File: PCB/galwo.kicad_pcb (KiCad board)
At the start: 2 copper layers, 20 parts, among them J1 Conn_02x20_Odd_Even, J2 Screw_Terminal_01x02, J3 Screw_Terminal_01x02, J4 Screw_Terminal_01x02, J5 Screw_Terminal_01x02, J6 Screw_Terminal_01x02, J7 Screw_Terminal_01x02, P1 Conn_01x03, U1 MCP4922, U2 MCP4922, U3 MCP4922, U4 TL074, U5 TL074, U6 TL074, U7 TL074

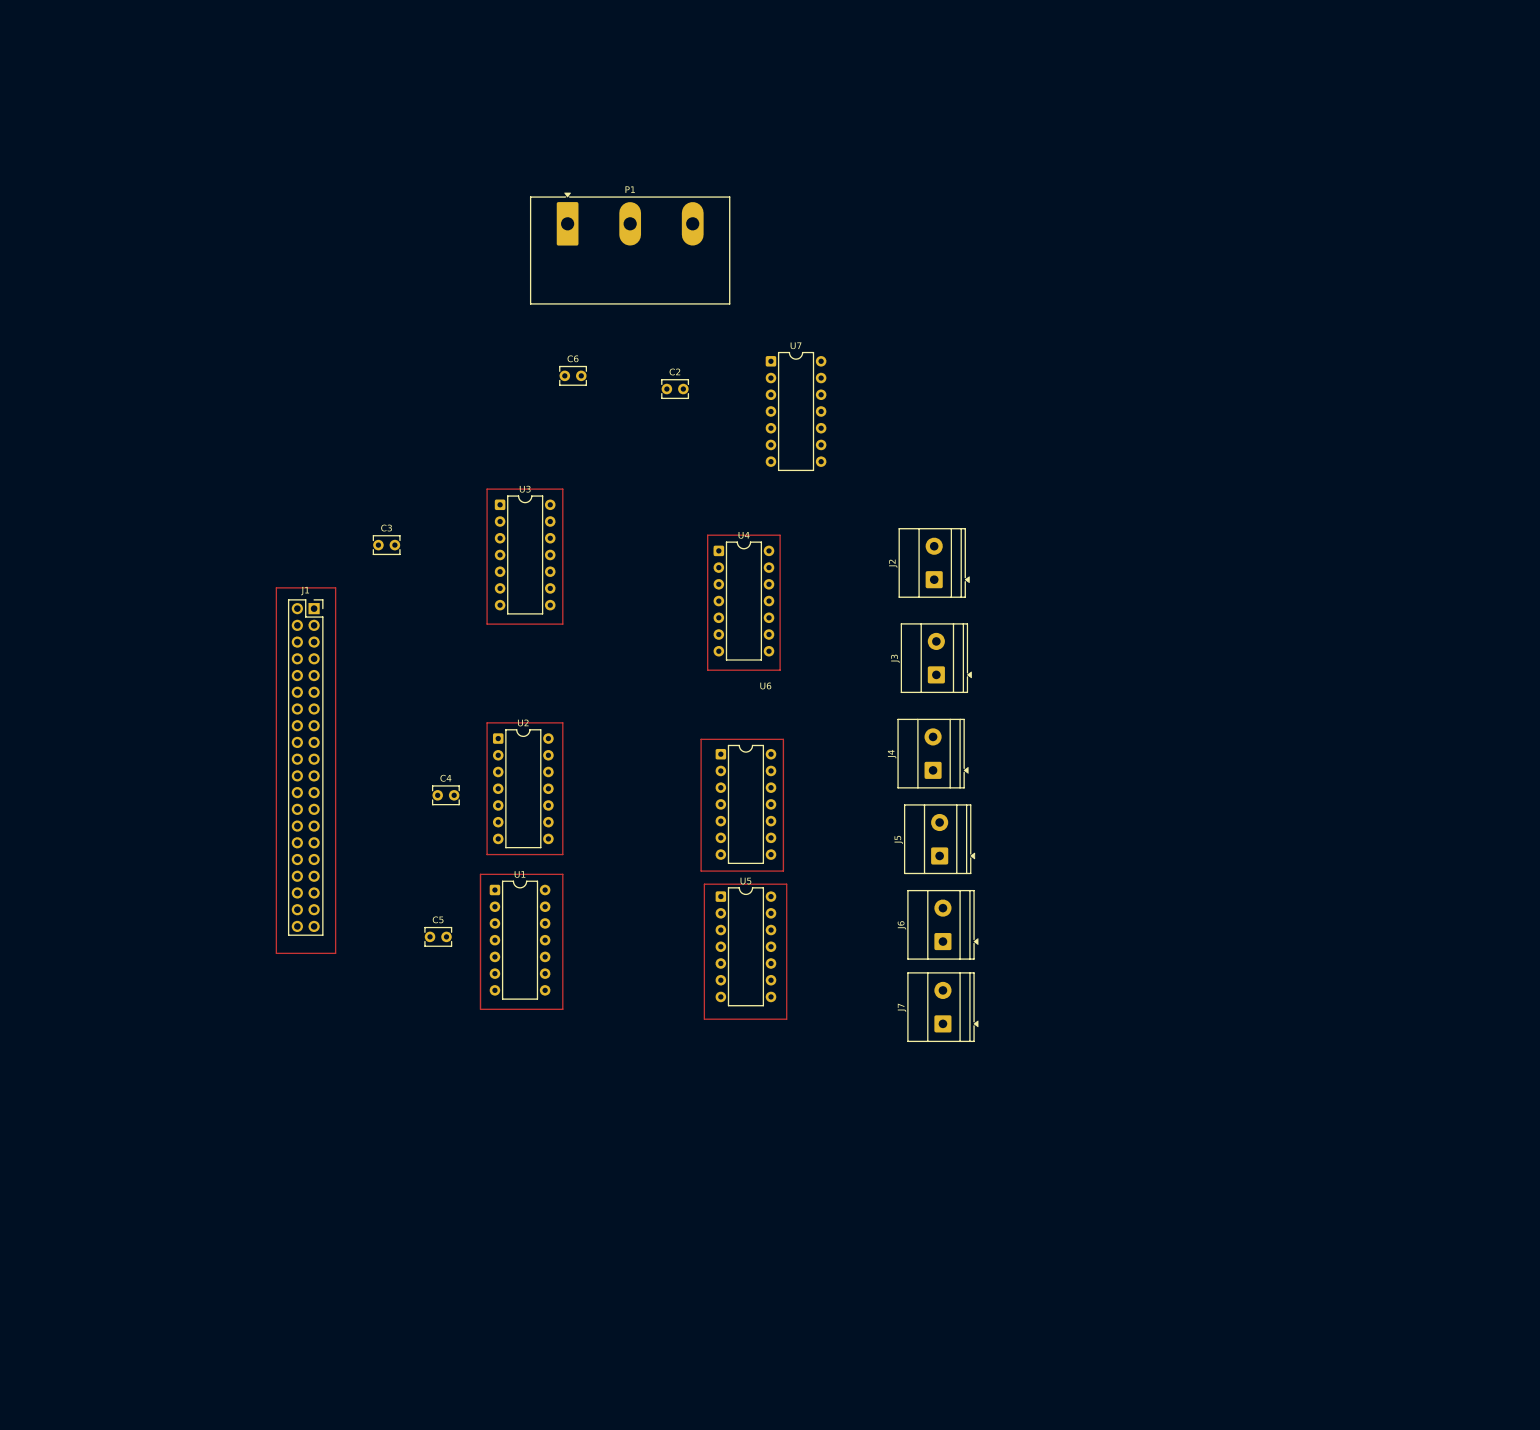
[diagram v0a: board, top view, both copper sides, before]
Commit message: Add files via upload
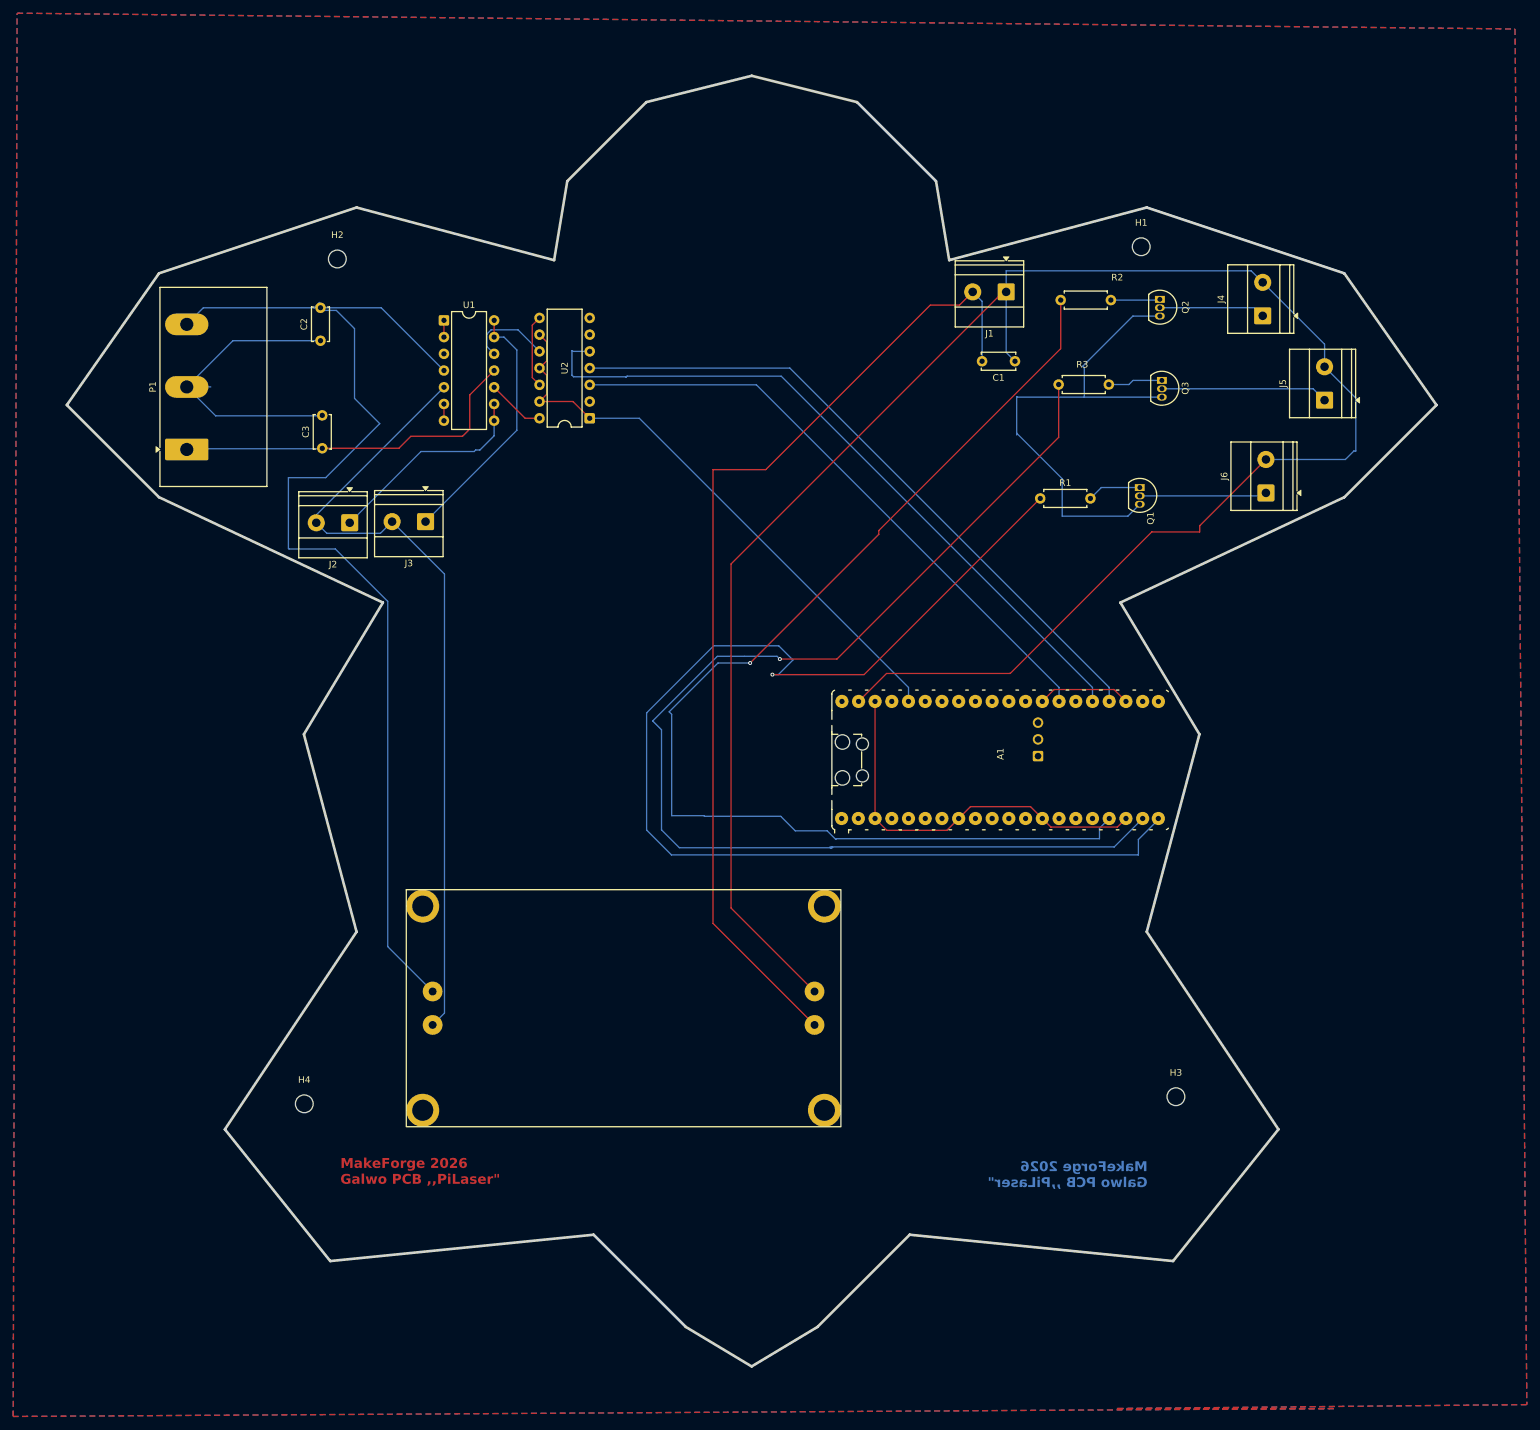
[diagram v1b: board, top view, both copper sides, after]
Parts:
- removed C4, C5, C6: 100nF, Capacitor_THT:C_Disc_D3.8mm_W2.6mm_P2.50mm
- removed U3: MCP4922, Package_DIP:DIP-14_W7.62mm
- removed U4, U5, U6, U7: TL074, Package_DIP:DIP-14_W7.62mm
- added A1: RaspberryPi_Pico_W, proba:RaspberryPi_Pico_W_SMD_HandSolder_tht, F.Cu at (149.7, 112.9)
- added C1: 100nF, Capacitor_THT:C_Disc_D5.0mm_W2.5mm_P5.00mm, F.Cu at (151.9, 52.4)
- added H1: MountingHole, MountingHole:MountingHole_2.7mm_M2.5, F.Cu at (171.1, 35.0)
- added H2: MountingHole, MountingHole:MountingHole_2.7mm_M2.5, F.Cu at (49.0, 36.8)
- added H3: MountingHole, MountingHole:MountingHole_2.7mm_M2.5, F.Cu at (176.4, 164.1)
- added H4: MountingHole, MountingHole:MountingHole_2.7mm_M2.5, F.Cu at (44.0, 165.1)
- added Q1: Q_NPN_BCE, Package_TO_SOT_THT:TO-92L_Inline, F.Cu at (170.9, 71.5)
- added Q2: Q_NPN_BCE, Package_TO_SOT_THT:TO-92L_Inline, F.Cu at (173.9, 43.0)
- added Q3: Q_NPN_BCE, Package_TO_SOT_THT:TO-92L_Inline, F.Cu at (174.2, 55.3)
- added R1: 1k, Resistor_THT:R_Axial_DIN0207_L6.3mm_D2.5mm_P7.62mm_Horizontal, F.Cu at (155.8, 73.2)
- added R2: 1k, Resistor_THT:R_Axial_DIN0207_L6.3mm_D2.5mm_P7.62mm_Horizontal, F.Cu at (158.9, 43.1)
- added R3: 1k, Resistor_THT:R_Axial_DIN0207_L6.3mm_D2.5mm_P7.62mm_Horizontal, F.Cu at (158.6, 55.9)
- C2, C3: footprint Capacitor_THT:C_Disc_D3.8mm_W2.6mm_P2.50mm -> Capacitor_THT:C_Disc_D5.0mm_W2.5mm_P5.00mm
- J1: value Conn_02x20_Odd_Even -> Conn_01x02; footprint Connector_PinSocket_2.54mm:PinSocket_2x20_P2.54mm_Vertical -> TerminalBlock_Phoenix:TerminalBlock_Phoenix_MKDS-1,5-2-5.08_1x02_P5.08mm_Horizontal
- J7: value Screw_Terminal_01x02 -> Conn_02x02_Counter_Clockwise; footprint TerminalBlock_Phoenix:TerminalBlock_Phoenix_MKDS-1,5-2-5.08_1x02_P5.08mm_Horizontal -> proba:Bez_nazwy
- U1: value MCP4922 -> TL074
- moved J1 115.6 mm to (150.6, 41.8), turned to 180 degrees
- moved J5 90.6 mm to (199.0, 58.3)
- moved J2 89.2 mm to (50.9, 76.9), turned to 180 degrees
- moved U1 86.9 mm to (65.2, 46.2)
- moved J4 85.3 mm to (189.6, 45.5)
- moved J6 83.9 mm to (190.1, 72.4)
- moved J3 81.0 mm to (62.4, 76.7), turned to 180 degrees
- moved P1 67.2 mm to (26.2, 65.8), turned to 90 degrees
- moved C2 53.1 mm to (46.5, 49.2), turned to 90 degrees
- moved U2 50.6 mm to (87.4, 61.0), turned to 180 degrees
- moved J7 48.6 mm to (92.5, 150.6), turned to 0 degrees
- moved C3 17.0 mm to (46.7, 65.6), turned to 90 degrees
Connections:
- C2 pad 1: Net-(J1-Pin_1) -> GND
- C2 pad 2: Net-(J1-Pin_6) -> /15V
- C3 pad 1: Net-(J1-Pin_1) -> /-15V
- C3 pad 2: Net-(J1-Pin_6) -> GND
- J1 pad 1: Net-(J1-Pin_1) -> Net-(A1-VSYS)
- J1 pad 2: unconnected-(J1-Pin_2-Pad2) -> GND
- J2 pad 2: Net-(J1-Pin_6) -> GND
- J3 pad 2: Net-(J1-Pin_6) -> GND
- J4 pad 2: Net-(J1-Pin_6) -> Net-(A1-VSYS)
- J5 pad 2: Net-(J1-Pin_6) -> Net-(A1-VSYS)
- J6 pad 2: Net-(J1-Pin_6) -> Net-(A1-VSYS)
- J7 pad 1: Net-(J7-Pin_1) -> GND
- J7 pad 2: Net-(J1-Pin_6) -> /15V
- P1 pad 1: Net-(P1-Pin_1) -> /-15V
- P1 pad 2: Net-(J1-Pin_6) -> GND
- P1 pad 3: Net-(P1-Pin_3) -> /15V
- U1 pad 1: Net-(J1-Pin_1) -> Net-(U1A--)
- U1 pad 10: Net-(U1-VB) -> Net-(U1C-+)
- U1 pad 11: Net-(J1-Pin_1) -> /-15V
- U1 pad 12: Net-(J1-Pin_6) -> Net-(U1D-+)
- U1 pad 13: Net-(J1-Pin_1) -> Net-(J3-Pin_1)
- U1 pad 14: Net-(U1-VA) -> Net-(J3-Pin_1)
- U1 pad 2: unconnected-(U1-NC-Pad2) -> Net-(U1A--)
- U1 pad 3: Net-(J1-Pin_26) -> GND
- U1 pad 4: Net-(J1-Pin_23) -> /15V
- U1 pad 5: Net-(J1-Pin_19) -> GND
- U1 pad 6: unconnected-(U1-NC-Pad6) -> Net-(U1B--)
- U1 pad 7: unconnected-(U1-NC-Pad7) -> Net-(U1B--)
- U1 pad 8: Net-(J1-Pin_6) -> Net-(J2-Pin_1)
- U1 pad 9: Net-(J1-Pin_1) -> Net-(J2-Pin_1)
- U2 pad 1: Net-(J1-Pin_1) -> Net-(A1-3V3)
- U2 pad 10: Net-(U2-VB) -> Net-(U1D-+)
- U2 pad 11: Net-(J1-Pin_1) -> Net-(A1-3V3)
- U2 pad 12: Net-(J1-Pin_6) -> GND
- U2 pad 13: Net-(J1-Pin_1) -> Net-(A1-3V3)
- U2 pad 14: Net-(U2-VA) -> Net-(U1C-+)
- U2 pad 3: Net-(J1-Pin_28) -> Net-(A1-GPIO21)
- U2 pad 4: Net-(J1-Pin_23) -> Net-(A1-GPIO18)
- U2 pad 5: Net-(J1-Pin_19) -> Net-(A1-GPIO19)
- U2 pad 8: Net-(J1-Pin_6) -> GND
- U2 pad 9: Net-(J1-Pin_1) -> Net-(A1-3V3)
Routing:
- net GND: track 0.00 -> 484.6 mm
- net Net-(A1-VSYS): track 0.00 -> 306.3 mm
- net Net-(A1-GPIO15): track 0.00 -> 184.0 mm, vias 0 -> 1
- net Net-(A1-GPIO14): track 0.00 -> 181.8 mm, vias 0 -> 1
- net Net-(A1-GPIO13): track 0.00 -> 176.1 mm, vias 0 -> 1
- net /15V: track 0.00 -> 176.0 mm
- net Net-(A1-GPIO19): track 0.00 -> 107.4 mm
- net Net-(A1-GPIO18): track 0.00 -> 101.1 mm
- net Net-(A1-GPIO21): track 0.00 -> 92.4 mm
- net Net-(A1-3V3): track 0.00 -> 88.1 mm
- net /-15V: track 0.00 -> 54.7 mm
- net Net-(J3-Pin_1): track 0.00 -> 38.6 mm
- net Net-(J2-Pin_1): track 0.00 -> 32.2 mm
- net Net-(J5-Pin_1): track 0.00 -> 25.4 mm
- net Net-(J6-Pin_1): track 0.00 -> 19.3 mm
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- added copper zone on B.Cu, net GND
- added copper zone on F.Cu, net GND
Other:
- board outline added: 208 x 196 mm
- board text added: "Blue"
- board text added: "Green"
- board text added: "MakeForge 2026 Galwo PCB ,,PiLaser{dblquote}"
- board text added: "Os X"
- board text added: "Os Y"
- board text added: "Red"
